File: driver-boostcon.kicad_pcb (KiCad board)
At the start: 2 copper layers, 100 x 80 mm, 63 parts, among them J301 Fuse Bypass, P301 On Switch, P302 Vcc, P303 PowerGND, P304 RegulatedPWR, P305 RegulatedGND, P601 Programmer, Q401 IRFH7084, Q402 BSC016N04LS, SW601 SW_Push, U601 ATMEGA328P-PU, U801 LM358, Y601 16 MHz

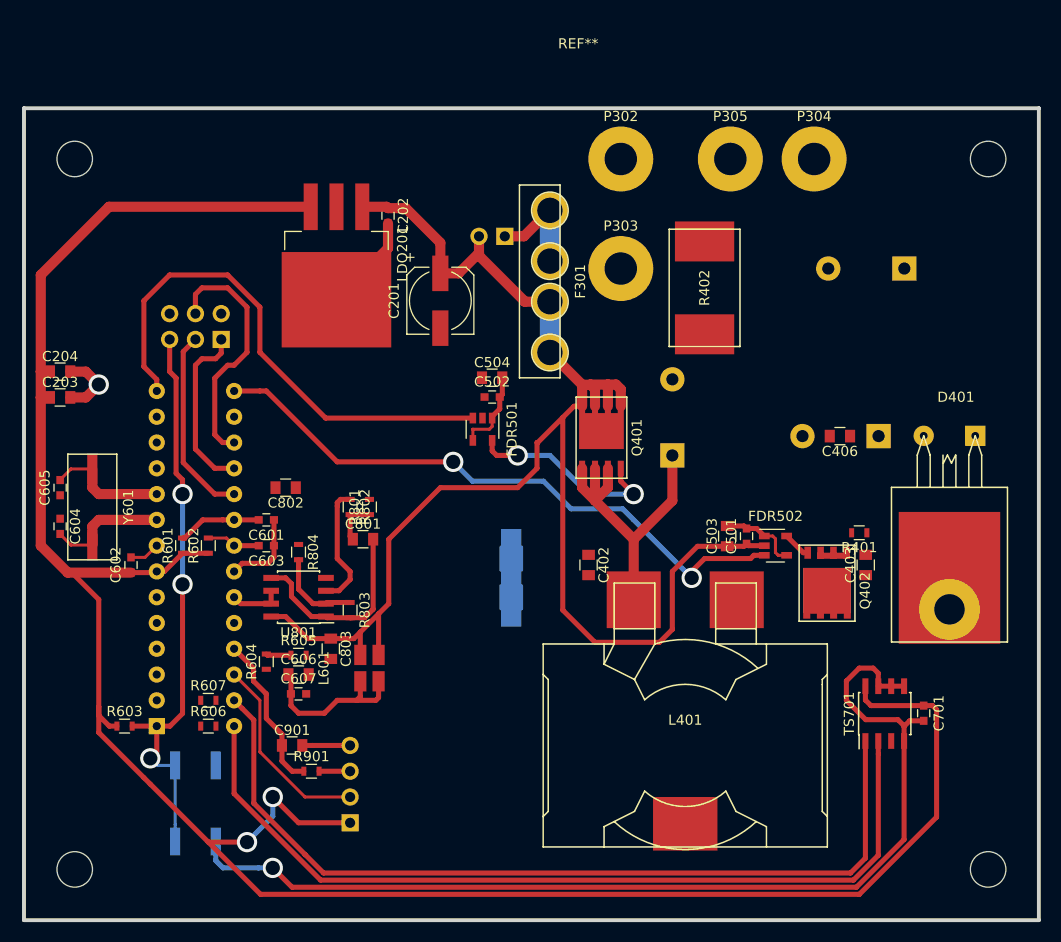
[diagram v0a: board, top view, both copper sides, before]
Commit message: Syncing
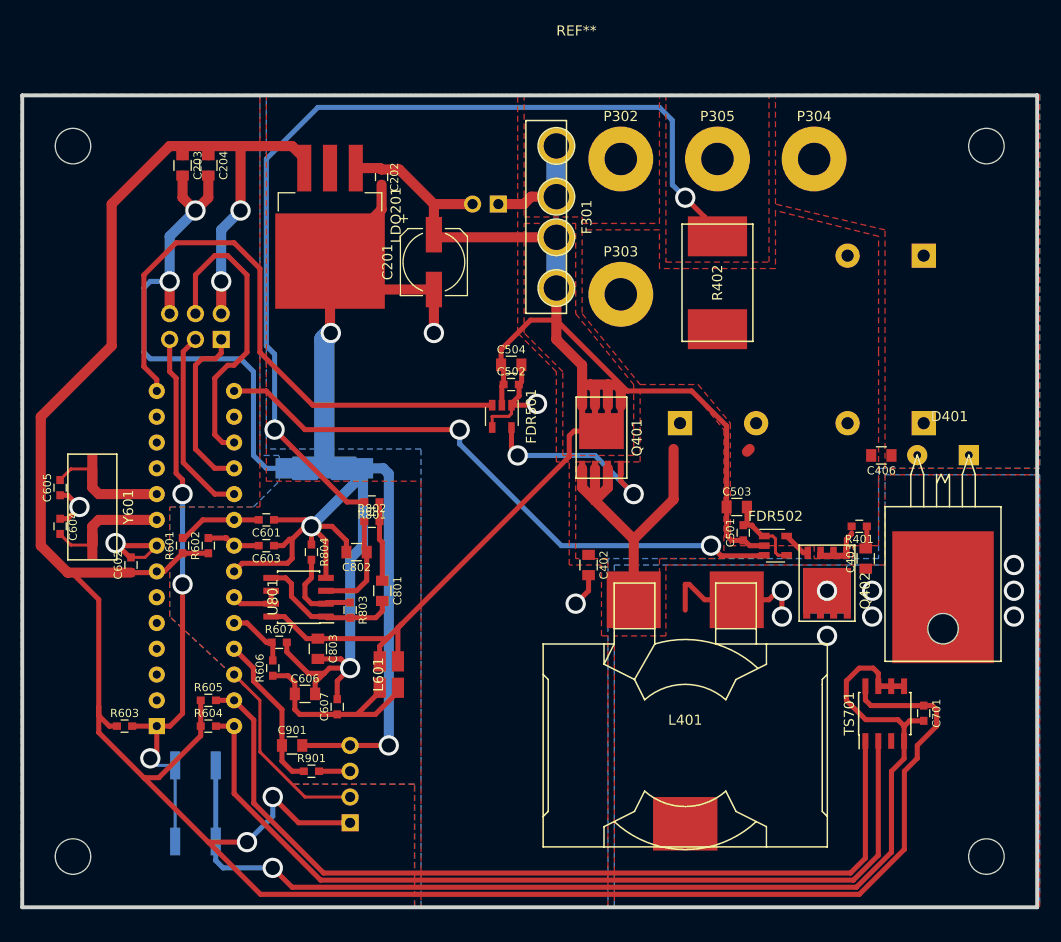
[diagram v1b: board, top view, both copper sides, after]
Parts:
- C202, C501, C502, C601, C602, C603, C604, C605, C607, C701: footprint Capacitors_SMD:C_0603 -> axel:C_0603_CustomText
- C203, C204, C402, C403, C406, C503, C504, C606, C801, C802, C803, C901: footprint Capacitors_SMD:C_0805 -> axel:C_0805_CustomText
- R401, R601, R602, R603, R604, R605, R606, R607, R801, R802, R803, R804, R901: footprint Resistors_SMD:R_0603 -> axel:C_0603_CustomText
- moved C203 25.8 mm to (63.5, 64.1), turned to 270 degrees
- moved C204 25.0 mm to (66.0, 64.1), turned to 270 degrees
- moved GND301 21.3 mm to (77.5, 94.0), turned to 180 degrees
- moved R605 9.94 mm to (66.0, 116.8)
- moved C802 9.44 mm to (80.6, 102.2)
- moved R607 9.03 mm to (73.0, 111.1)
- moved R604 8.54 mm to (66.0, 119.4), turned to 0 degrees
- moved R606 8.54 mm to (72.4, 113.7), turned to 90 degrees
- moved F301 6.38 mm to (100.3, 69.2)
- moved C801 5.43 mm to (83.2, 106.0), turned to 270 degrees
- moved C404 4.62 mm to (136.5, 89.5)
- moved C406 4.50 mm to (132.3, 92.7)
- moved C607 4.02 mm to (78.7, 117.5), turned to 90 degrees
- moved C201 3.86 mm to (88.3, 73.7)
- moved LDO201 3.86 mm to (78.0, 69.0)
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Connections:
- net Net-(C401-Pad1) renamed /Power stage/PowerVcc
- net Net-(C601-Pad2) renamed /MCU/AVcc
- net Net-(C603-Pad2) renamed /MCU/AREF
- net Net-(R606-Pad2) renamed /MCU/Vsense
- GND301 pad 1: GNDPWR -> GNDREF
- GND301 pad 2: GNDREF -> GNDPWR
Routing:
- net GNDREF: track 12.9 -> 113.1 mm, vias 0 -> 3
- net /CurrentSense/CurrentSignal: track 0.00 -> 94.7 mm, vias 0 -> 2
- net GNDD: track 112.3 -> 178.5 mm, vias 2 -> 5
- net GNDPWR: track 29.9 -> 74.4 mm, vias 0 -> 4
- net +5C: track 226.4 -> 257.8 mm, vias 2 -> 4
- net /Power stage/SwitchNode: track 0.00 -> 15.5 mm, vias 0 -> 3
- net /MCU/PowerDriveSignal: track 51.3 -> 59.1 mm
- net VCC: track 143.8 -> 150.3 mm
- net /MCU/Vsense: track 0.00 -> 6.32 mm
- net /MCU/MOSI: track 24.5 -> 30.1 mm
- net Net-(C801-Pad2): track 19.9 -> 14.8 mm
- net Net-(C606-Pad1): track 16.4 -> 20.5 mm
- net Net-(C801-Pad1): track 4.44 -> 7.86 mm
- net Net-(C403-Pad2): track 0.00 -> 2.22 mm
- net Net-(C802-Pad1): track 12.3 -> 10.4 mm
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- added copper zone on F.Cu, net /CurrentSense/CurrentSignal
- added copper zone on F.Cu, net /Power stage/PowerRegulated
- added copper zone on F.Cu, net /Power stage/PowerVcc
- added copper zone on B.Cu, net /Power stage/SwitchNode
- added copper zone on F.Cu, net /Power stage/SwitchNode
- added copper zone on B.Cu, net GNDD
- added copper zone on F.Cu, net GNDD
- added copper zone on B.Cu, net GNDPWR
- added copper zone on F.Cu, net GNDPWR
- added copper zone on F.Cu, net Net-(F301-Pad2)
- added copper zone on F.Cu, net VCC
